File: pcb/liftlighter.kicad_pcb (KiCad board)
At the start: 2 copper layers, 60 x 90 mm, 55 parts, among them IC1 ATMEGA8-P, P1 CONN_01X06, P12 CONN_01X02, P2 CONN_02X10, P3 CONN_01X02, Q1 BC548, Q10 BC548, Q2 BC548, Q3 BC548, Q4 BC548, Q5 BC548, Q6 BC548, Q7 BC548, Q8 BC548, Q9 BC548, SW1 SW_PUSH, SW2 SW_PUSH, U1 LD1117S33TR, Y1 Crystal

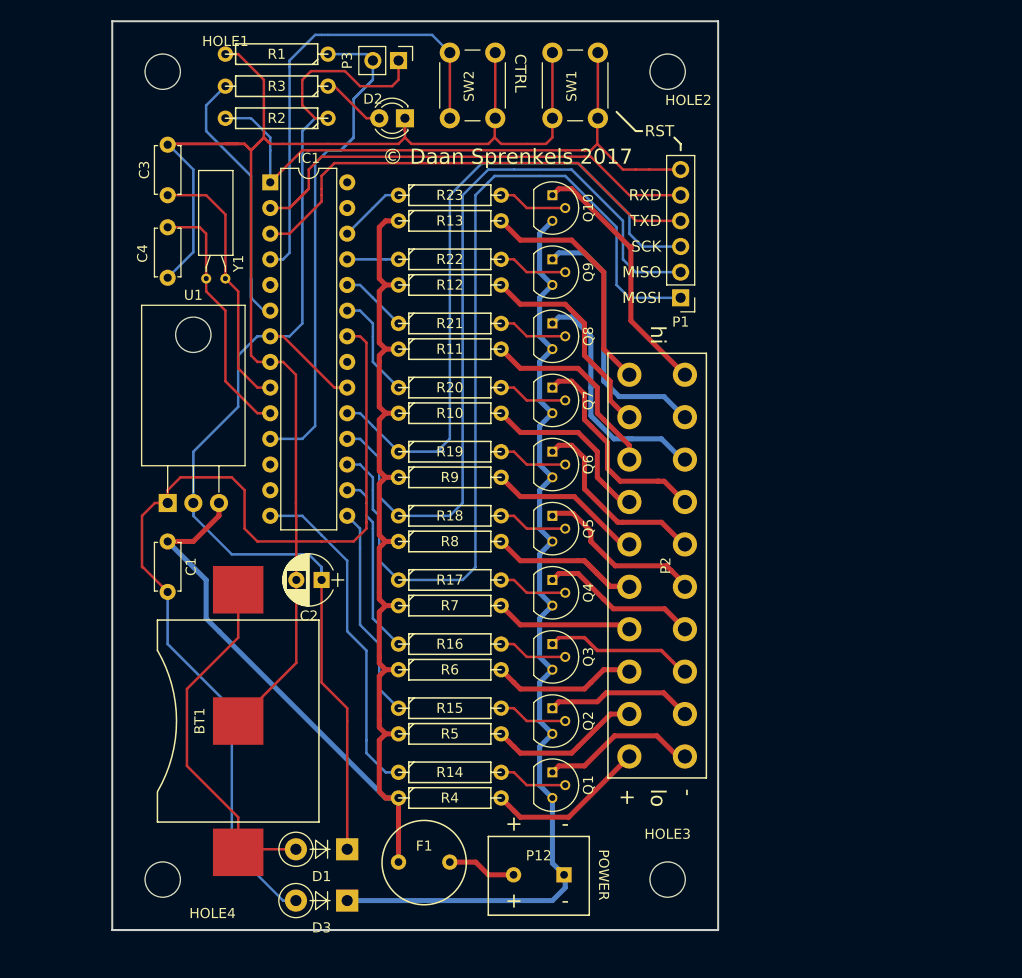
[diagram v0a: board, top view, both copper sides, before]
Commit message: Backup time every day
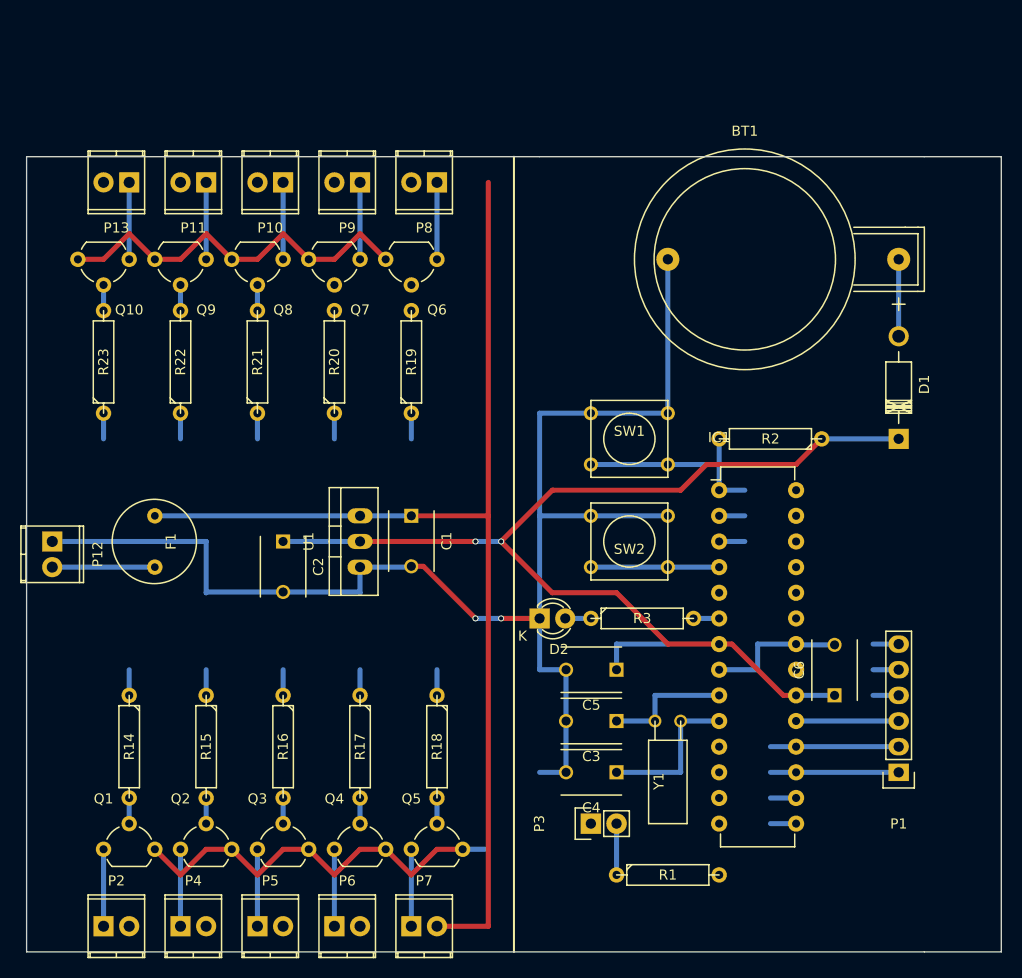
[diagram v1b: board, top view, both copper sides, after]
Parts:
- removed D3: D, Diodes_ThroughHole:D_DO-41_SOD81_P5.08mm_Vertical_KathodeUp
- removed HOLE1, HOLE2, HOLE3, HOLE4: MountingHole_3.5mm, Mounting_Holes:MountingHole_3.5mm
- removed R10, R11, R12, R13, R4, R5, R6, R7, R8, R9: R, Discret:R4
- added C5: 100nF, Capacitors_ThroughHole:C_Disc_D6_P5, F.Cu at (154.9, 109.2)
- added C6: 100nF, Capacitors_ThroughHole:C_Disc_D6_P5, F.Cu at (176.5, 111.8)
- added P10: CONN_01X02, Terminal_Blocks:TerminalBlock_Pheonix_MPT-2.54mm_2pol, F.Cu at (121.9, 61.0)
- added P11: CONN_01X02, Terminal_Blocks:TerminalBlock_Pheonix_MPT-2.54mm_2pol, F.Cu at (114.3, 61.0)
- added P13: CONN_01X02, Terminal_Blocks:TerminalBlock_Pheonix_MPT-2.54mm_2pol, F.Cu at (106.7, 61.0)
- added P4: CONN_01X02, Terminal_Blocks:TerminalBlock_Pheonix_MPT-2.54mm_2pol, F.Cu at (111.8, 134.6)
- added P5: CONN_01X02, Terminal_Blocks:TerminalBlock_Pheonix_MPT-2.54mm_2pol, F.Cu at (119.4, 134.6)
- added P6: CONN_01X02, Terminal_Blocks:TerminalBlock_Pheonix_MPT-2.54mm_2pol, F.Cu at (127.0, 134.6)
- added P7: CONN_01X02, Terminal_Blocks:TerminalBlock_Pheonix_MPT-2.54mm_2pol, F.Cu at (134.6, 134.6)
- added P8: CONN_01X02, Terminal_Blocks:TerminalBlock_Pheonix_MPT-2.54mm_2pol, F.Cu at (137.2, 61.0)
- added P9: CONN_01X02, Terminal_Blocks:TerminalBlock_Pheonix_MPT-2.54mm_2pol, F.Cu at (129.5, 61.0)
- BT1: footprint CUSTOM:RENATA100340 -> Connect:CR2032H
- C1, C3, C4: footprint Capacitors_ThroughHole:C_Disc_D4.7mm_W2.5mm_P5.00mm -> Capacitors_ThroughHole:C_Disc_D6_P5
- C2: footprint Capacitors_ThroughHole:CP_Radial_D5.0mm_P2.50mm -> Capacitors_ThroughHole:C_Disc_D6_P5
- D1: footprint Diodes_ThroughHole:D_DO-41_SOD81_P5.08mm_Vertical_KathodeUp -> Diodes_ThroughHole:Diode_DO-41_SOD81_Horizontal_RM10
- D2: footprint LEDs:LED_D3.0mm -> LEDs:LED-3MM
- P1: footprint Pin_Headers:Pin_Header_Straight_1x06_Pitch2.54mm -> Pin_Headers:Pin_Header_Straight_1x06
- P12: footprint CUSTOM:DG126-5.0-02P-14-00AH -> Terminal_Blocks:TerminalBlock_Pheonix_MPT-2.54mm_2pol
- P2: value CONN_02X10 -> CONN_01X02; footprint CUSTOM:TE2-1586037-0 -> Terminal_Blocks:TerminalBlock_Pheonix_MPT-2.54mm_2pol
- P3: footprint Pin_Headers:Pin_Header_Straight_1x02_Pitch2.54mm -> Pin_Headers:Pin_Header_Straight_1x02
- Q1, Q10, Q2, Q3, Q4, Q5, Q6, Q7, Q8, Q9: footprint TO_SOT_Packages_THT:TO-92_Molded_Narrow -> TO_SOT_Packages_THT:TO-92_Molded_Wide
- R1: value R -> 50K
- R3: value R -> 160
- SW1, SW2: footprint Buttons_Switches_ThroughHole:SW_PUSH_6mm -> Buttons_Switches_ThroughHole:SW_PUSH_SMALL
- U1: footprint TO_SOT_Packages_THT:TO-220_Horizontal -> TO_SOT_Packages_THT:TO-220_Neutral123_Vertical
- Y1: footprint Crystals:Crystal_C38-LF_d3.0mm_l8.0mm_Horizontal -> Crystals:Crystal_Watch
- moved R1 90.0 mm to (160.0, 129.5), turned to 0 degrees
- moved P3 77.9 mm to (152.4, 124.5), turned to 90 degrees
- moved P2 75.5 mm to (104.1, 134.6), turned to 0 degrees
- moved C4 69.9 mm to (154.9, 119.4), turned to 180 degrees
- moved C3 68.5 mm to (154.9, 114.3), turned to 180 degrees
- moved D1 68.1 mm to (182.9, 86.4), turned to 90 degrees
- moved BT1 67.9 mm to (167.6, 68.6), turned to 0 degrees
- moved R3 63.9 mm to (157.5, 104.1), turned to 0 degrees
- moved Y1 62.0 mm to (160.0, 114.3), turned to 0 degrees
- moved R2 58.3 mm to (170.2, 86.4)
- moved IC1 53.9 mm to (165.1, 91.4)
- moved P12 52.1 mm to (99.1, 96.5), turned to 270 degrees
- moved P1 51.7 mm to (182.9, 119.4)
- moved D2 51.3 mm to (147.3, 104.1), turned to 0 degrees
- moved SW2 45.5 mm to (156.2, 96.5), turned to 180 degrees
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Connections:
- IC1 pad 12: Net-(IC1-Pad12) -> (no net)
- IC1 pad 13: Net-(IC1-Pad13) -> (no net)
- IC1 pad 21: Net-(IC1-Pad21) -> (no net)
- IC1 pad 27: Net-(IC1-Pad27) -> (no net)
- IC1 pad 28: Net-(IC1-Pad28) -> (no net)
- IC1 pad 5: Net-(IC1-Pad5) -> (no net)
- P12 pad 1: -12VA -> GND
- P2 pad 2: Net-(P2-Pad2) -> +12V
- Q1 pad 1: Net-(P2-Pad20) -> Net-(P2-Pad1)
- Q1 pad 3: -12VA -> GND
- Q10 pad 1: Net-(P2-Pad2) -> Net-(P13-Pad1)
- Q10 pad 3: -12VA -> GND
- Q2 pad 1: Net-(P2-Pad18) -> Net-(P4-Pad1)
- Q2 pad 3: -12VA -> GND
- Q3 pad 1: Net-(P2-Pad16) -> Net-(P5-Pad1)
- Q3 pad 3: -12VA -> GND
- Q4 pad 1: Net-(P2-Pad14) -> Net-(P6-Pad1)
- Q4 pad 3: -12VA -> GND
- Q5 pad 1: Net-(P2-Pad12) -> Net-(P7-Pad1)
- Q5 pad 3: -12VA -> GND
- Q6 pad 1: Net-(P2-Pad10) -> Net-(P8-Pad1)
- Q6 pad 3: -12VA -> GND
- Q7 pad 1: Net-(P2-Pad8) -> Net-(P9-Pad1)
- Q7 pad 3: -12VA -> GND
- Q8 pad 1: Net-(P2-Pad6) -> Net-(P10-Pad1)
- Q8 pad 3: -12VA -> GND
- Q9 pad 1: Net-(P2-Pad4) -> Net-(P11-Pad1)
- Q9 pad 3: -12VA -> GND
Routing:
- net -12VA: track 98.3 -> 0.00 mm
- net /a3: track 88.7 -> 15.2 mm
- net /a4: track 76.9 -> 15.2 mm
- net /a5: track 66.4 -> 12.7 mm
- net Net-(IC1-Pad11): track 54.7 -> 5.08 mm
- net Net-(IC1-Pad2): track 48.1 -> 5.08 mm
- net Net-(IC1-Pad3): track 48.0 -> 5.08 mm
- net Net-(IC1-Pad1): track 62.1 -> 22.9 mm
- net Net-(IC1-Pad4): track 45.5 -> 12.7 mm
- net /a0: track 33.3 -> 2.54 mm
- net Net-(BT1-Pad1): track 36.0 -> 7.62 mm
- net Net-(P2-Pad4): track 26.4 -> 0.00 mm
- net Net-(P2-Pad2): track 25.9 -> 0.00 mm
- net Net-(IC1-Pad6): track 27.9 -> 2.54 mm
- net Net-(P2-Pad6): track 24.2 -> 0.00 mm
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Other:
- board size 60 x 90 mm -> 96.5 x 78.7 mm
- net class 12V removed
- net class Default: clearance 0.2 -> 0.25; trace_width 0.25 -> 0.5
- rule pad_to_mask_clearance: 0.2 -> 0
- rule trace_clearance: 0.2 -> 0.25
- board text removed: "+"
- board text removed: "-"
- board text removed: "CTRL"
- board text removed: "MISO"
- board text removed: "MOSI"
- board text removed: "POWER"
- board text removed: "RST"
- board text removed: "RXD"
- board text removed: "SCK"
- board text removed: "TXD"
- board text removed: "hi"
- board text removed: "lo"
- board text removed: "© Daan Sprenkels 2017"
